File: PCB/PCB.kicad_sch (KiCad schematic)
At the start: 5 parts, among them J1 Screw_Terminal_01x02, J2 Screw_Terminal_01x02, J3 Screw_Terminal_01x02, J4 Screw_Terminal_01x02

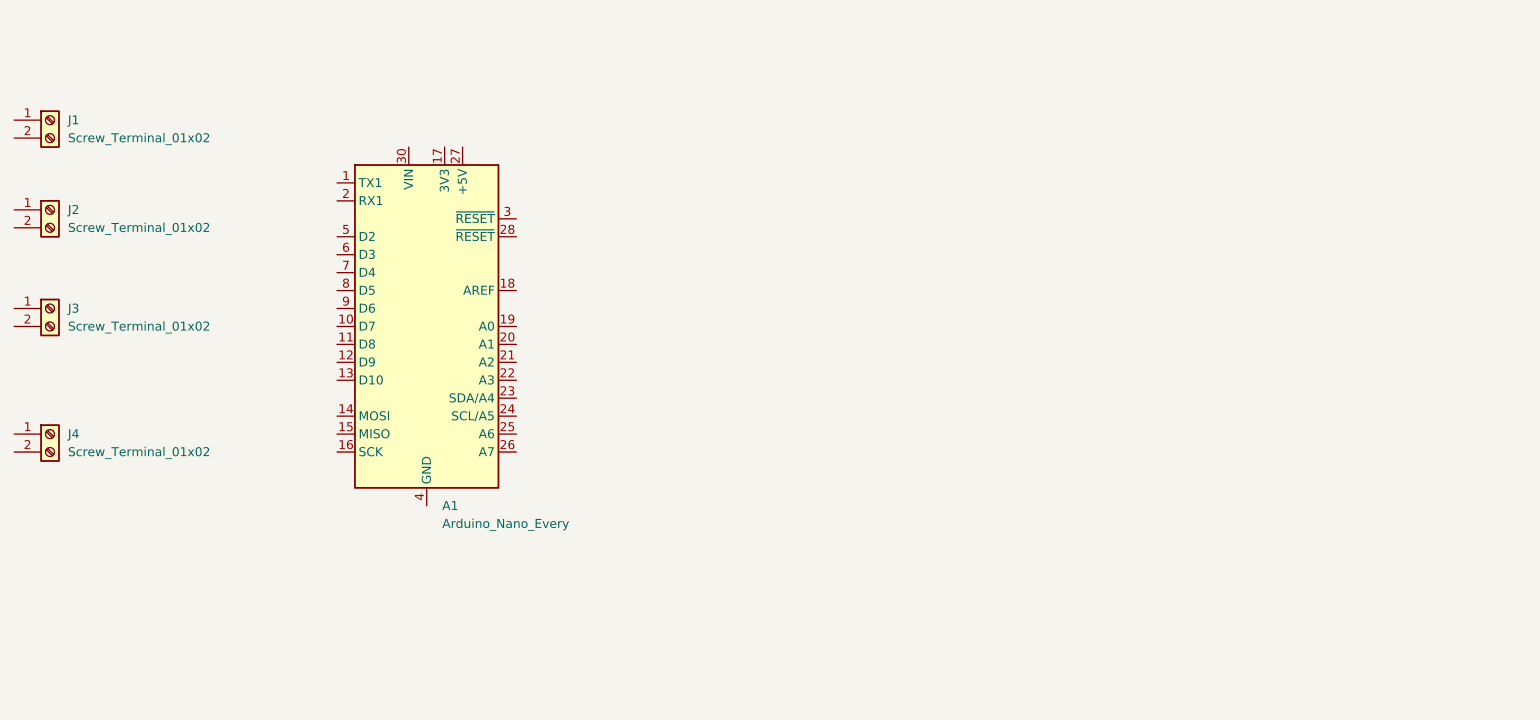
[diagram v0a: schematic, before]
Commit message: 28 del 1
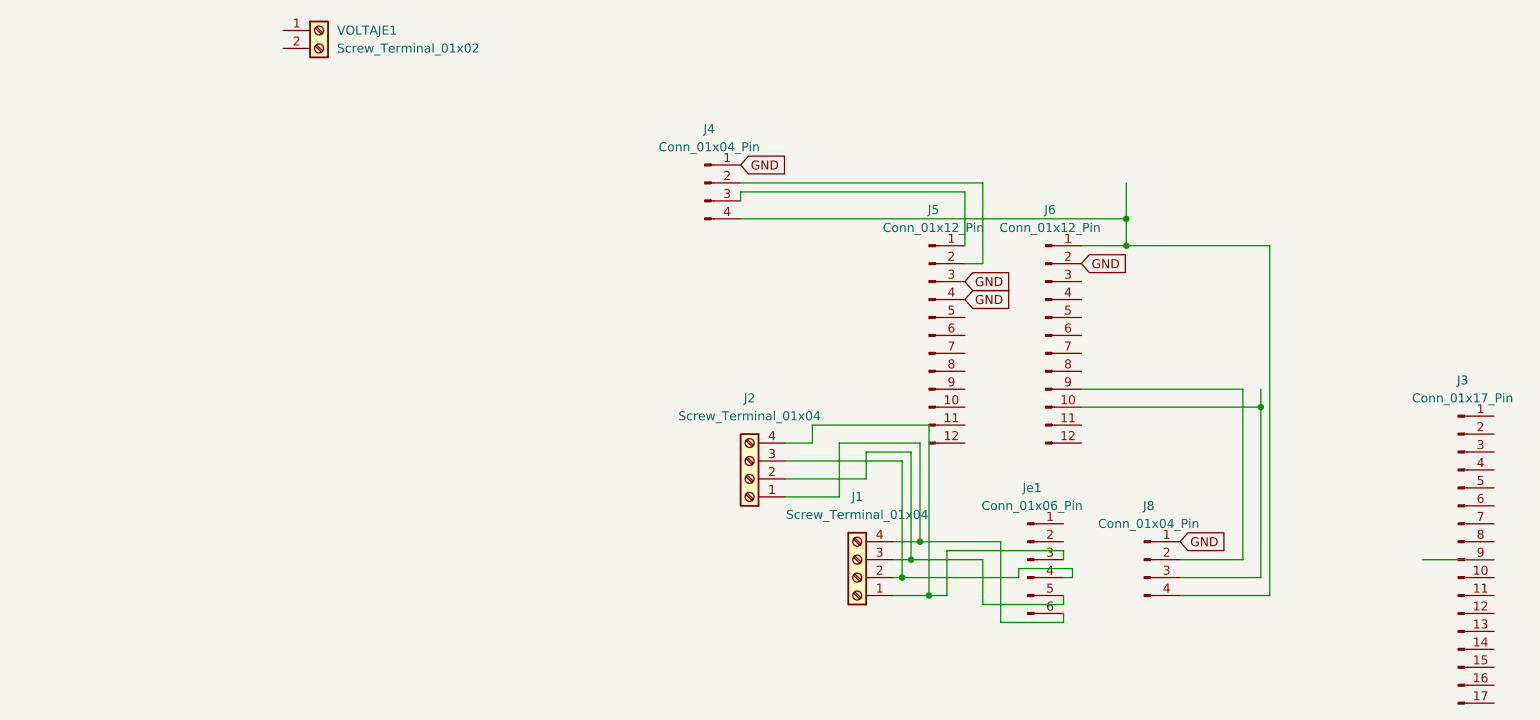
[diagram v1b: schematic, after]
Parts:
- removed A1: Arduino_Nano_Every, Module:Arduino_Nano, symbol MCU_Module:Arduino_Nano_Every
- removed J1, J2, J3, J4: Screw_Terminal_01x02, TerminalBlock:TerminalBlock_Xinya_XY308-2.54-2P_1x02_P2.54mm_Horizontal, symbol Connector:Screw_Terminal_01x02
- added J1, J2: Screw_Terminal_01x04, TerminalBlock:TerminalBlock_Altech_AK300-4_P5.00mm, symbol Connector:Screw_Terminal_01x04
- added J3: Conn_01x17_Pin, Connector_PinSocket_2.54mm:PinSocket_1x17_P2.54mm_Vertical, symbol Connector:Conn_01x17_Pin
- added J4: Conn_01x04_Pin, Connector_PinHeader_2.54mm:PinHeader_1x04_P2.54mm_Vertical, symbol Connector:Conn_01x04_Pin
- added J5, J6: Conn_01x12_Pin, Connector_PinSocket_2.54mm:PinSocket_1x12_P2.54mm_Vertical, symbol Connector:Conn_01x12_Pin
- added J8: Conn_01x04_Pin, Connector_PinSocket_2.54mm:PinSocket_1x04_P2.54mm_Vertical, symbol Connector:Conn_01x04_Pin
- added Je1: Conn_01x06_Pin, Connector_PinSocket_2.54mm:PinSocket_1x06_P2.54mm_Vertical, symbol Connector:Conn_01x06_Pin
- added VOLTAJE1: Screw_Terminal_01x02, TerminalBlock:TerminalBlock_Altech_AK300-2_P5.00mm, symbol Connector:Screw_Terminal_01x02
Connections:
- new net: J4.3 (Pin_3), J5.1 (Pin_1)
- new net: J4.2 (Pin_2), J5.2 (Pin_2)
- new net: J4.4 (Pin_4), J6.1 (Pin_1), J8.4 (Pin_4)
- new net: J6.10 (Pin_10), J8.3 (Pin_3)
- new net: J6.9 (Pin_9), J8.2 (Pin_2)
- new net: J1.1 (Pin_1), J2.4 (Pin_4), Je1.3 (Pin_3)
- new net: J1.2 (Pin_2), J2.3 (Pin_3), Je1.4 (Pin_4)
- new net: J1.3 (Pin_3), J2.2 (Pin_2), Je1.5 (Pin_5)
- new net: J1.4 (Pin_4), J2.1 (Pin_1), Je1.6 (Pin_6)
- new net GND: J4.1 (Pin_1), J5.3 (Pin_3), J5.4 (Pin_4), J6.2 (Pin_2), J8.1 (Pin_1)
